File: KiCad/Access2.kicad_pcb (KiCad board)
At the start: 2 copper layers, 50 x 26.5 mm, 65 parts, among them J1 USB-C, J2 RFID, J3 INPUTS, J4 ExtTamper, J5 POWER, J6 DOOR, Q1 NX7002AK, SW1 Tamper, U1 ESP32-PICO-MINI-02, U2 FT231XQ, U3 G3VM-41GR8, U4 LMR16006+FB, U5 LMR16006+FB, U6 AA, U7 QR

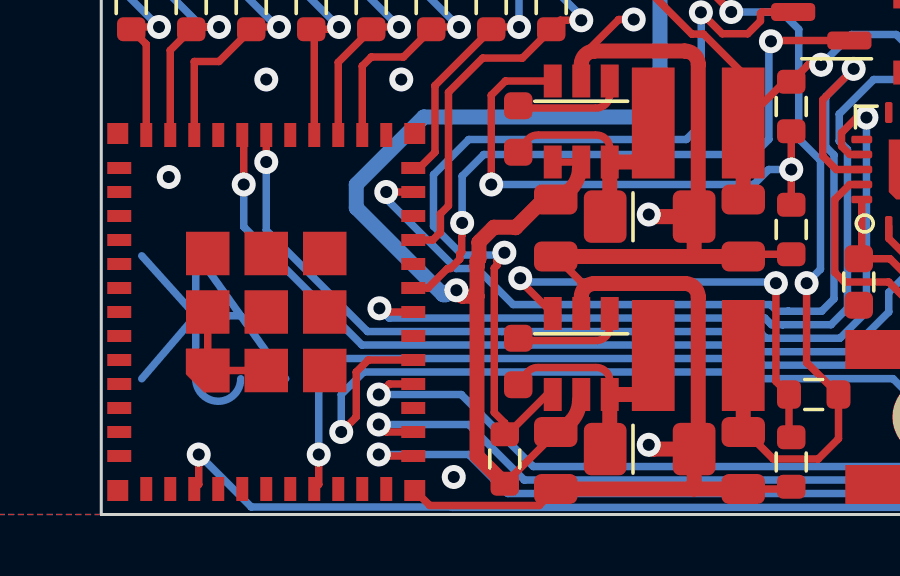
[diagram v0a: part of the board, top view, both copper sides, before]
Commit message: Tweak
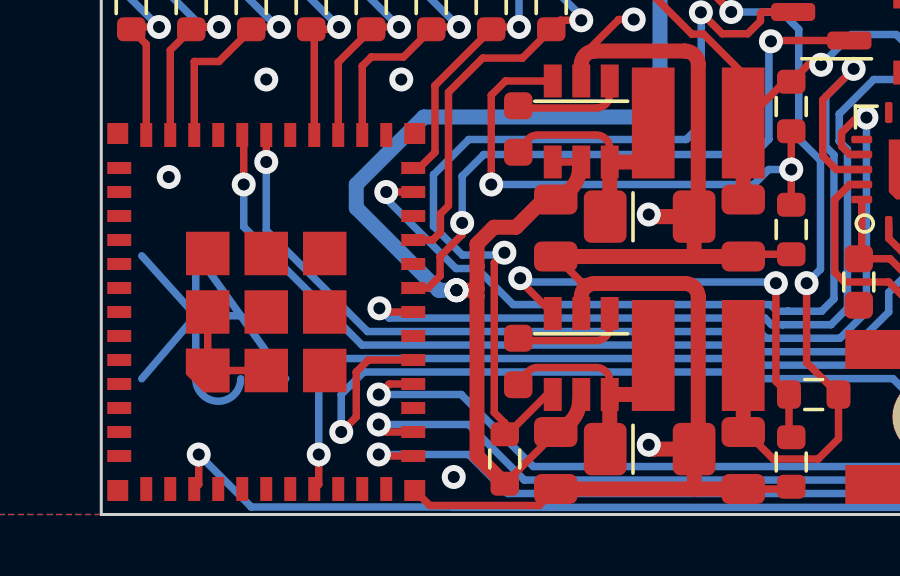
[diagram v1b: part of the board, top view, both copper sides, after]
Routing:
- net +12V: track 62.7 -> 62.5 mm, vias 1 -> 2
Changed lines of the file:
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@@
   (segment (start 128.620662 85.951956) (end 116.098352 85.951956) (width 0.25) (layer "B.Cu") (net 9))
   (segment (start 132.25 78) (end 131.098531 79.151469) (width 0.25) (layer "B.Cu") (net 9))
-  (segment (start 118.514852 83.746481) (end 118.514852 83.183896) (width 0.25) (layer "F.Cu") (net 10))
-  (segment (start 118.039296 84.300999) (end 118.136519 84.300999) (width 0.25) (layer "F.Cu") (net 10))
-  (segment (start 118.451458 83.809875) (end 118.514852 83.746481) (width 0.25) (layer "F.Cu") (net 10))
+  (segment (start 118.529927 82.779927) (end 118.529927 83.168821) (width 0.25) (layer "F.Cu") (net 10))
   (segment (start 131.4375 76.7) (end 128.849198 76.7) (width 0.25) (layer "F.Cu") (net 10))
-  (segment (start 118.451458 83.98606) (end 118.451458 83.809875) (width 0.25) (layer "F.Cu") (net 10))
-  (segment (start 116.9 84.95) (end 117.390295 84.95) (width 0.25) (layer "F.Cu") (net 10))
-  (segment (start 118.136519 84.300999) (end 118.451458 83.98606) (width 0.25) (layer "F.Cu") (net 10))
-  (segment (start 118.514852 83.183896) (end 118.529927 83.168821) (width 0.25) (layer "F.Cu") (net 10))
+  (segment (start 117.390295 84.95) (end 116.9 84.95) (width 0.25) (layer "F.Cu") (net 10))
   (segment (start 128.849198 76.7) (end 128.822959 76.726239) (width 0.25) (layer "F.Cu") (net 10))
-  (segment (start 118.529927 83.168821) (end 118.529927 82.779927) (width 0.25) (layer "F.Cu") (net 10))
-  (segment (start 117.390295 84.95) (end 118.039296 84.300999) (width 0.25) (layer "F.Cu") (net 10))
+  (segment (start 117.795148 84.545148) (end 117.390295 84.95) (width 0.25) (layer "F.Cu") (net 10))
+  (segment (start 117.795148 83.9036) (end 117.795148 84.545148) (width 0.25) (layer "F.Cu") (net 10))
+  (segment (start 118.529927 83.168821) (end 117.795148 83.9036) (width 0.25) (layer "F.Cu") (net 10))
   (via (at 128.822959 76.726239) (size 0.8) (drill 0.4) (layers "F.Cu" "B.Cu") (net 10))
   (via (at 118.529927 82.779927) (size 0.8) (drill 0.4) (layers "F.Cu" "B.Cu") (net 10))
@@
   (segment (start 131.727456 87.522544) (end 132.75 86.5) (width 0.25) (layer "B.Cu") (net 16))
   (segment (start 113.75 88) (end 114.44951 87.30049) (width 0.25) (layer "B.Cu") (net 16))
-  (segment (start 119.089363 83.984452) (end 119.025969 84.047846) (width 0.5) (layer "F.Cu") (net 17))
-  (segment (start 119.586988 82.924242) (end 119.089363 83.421867) (width 0.5) (layer "F.Cu") (net 17))
+  (segment (start 119.02548 84.97452) (end 119.02548 85.22452) (width 0.5) (layer "F.Cu") (net 17))
   (segment (start 142 76.75) (end 143.5125 76.75) (width 0.5) (layer "F.Cu") (net 17))
-  (segment (start 121.25 82) (end 120.308249 82.941751) (width 0.5) (layer "F.Cu") (net 17))
   (segment (start 143.5125 76.75) (end 144.7625 75.5) (width 0.5) (layer "F.Cu") (net 17))
-  (segment (start 119.02548 84.22452) (end 119.02548 85.22452) (width 0.5) (layer "F.Cu") (net 17))
-  (segment (start 118.538415 85.22452) (end 118.339395 85.0255) (width 0.5) (layer "F.Cu") (net 17))
+  (segment (start 119.025969 83.485261) (end 119.025969 84.224031) (width 0.5) (layer "F.Cu") (net 17))
+  (segment (start 118.339395 85.0255) (end 118.9745 85.0255) (width 0.5) (layer "F.Cu") (net 17))
+  (segment (start 120.325758 82.924242) (end 119.586988 82.924242) (width 0.5) (layer "F.Cu") (net 17))
+  (segment (start 119.586988 82.924242) (end 119.025969 83.485261) (width 0.5) (layer "F.Cu") (net 17))
+  (segment (start 118.9745 85.0255) (end 119.02548 84.97452) (width 0.5) (layer "F.Cu") (net 17))
+  (segment (start 119.025969 84.224031) (end 119.02548 84.22452) (width 0.5) (layer "F.Cu") (net 17))
   (segment (start 121.65 89.775) (end 119.95 91.475) (width 0.25) (layer "F.Cu") (net 17))
-  (segment (start 119.025969 84.224031) (end 119.02548 84.22452) (width 0.5) (layer "F.Cu") (net 17))
-  (segment (start 120.29074 82.924242) (end 119.586988 82.924242) (width 0.5) (layer "F.Cu") (net 17))
   (segment (start 121.65 82) (end 121.25 82) (width 0.5) (layer "F.Cu") (net 17))
   (segment (start 119.02548 90.55048) (end 119.95 91.475) (width 0.5) (layer "F.Cu") (net 17))
-  (segment (start 120.308249 82.941751) (end 120.29074 82.924242) (width 0.5) (layer "F.Cu") (net 17))
   (segment (start 121.55 80.75) (end 122.5 80.75) (width 0.25) (layer "F.Cu") (net 17))
   (segment (start 119.02548 85.22452) (end 119.02548 90.55048) (width 0.5) (layer "F.Cu") (net 17))
-  (segment (start 119.02548 85.22452) (end 118.538415 85.22452) (width 0.5) (layer "F.Cu") (net 17))
-  (segment (start 119.089363 83.421867) (end 119.089363 83.984452) (width 0.5) (layer "F.Cu") (net 17))
   (segment (start 121.65 89.75) (end 121.65 89.775) (width 0.25) (layer "F.Cu") (net 17))
-  (segment (start 119.025969 84.047846) (end 119.025969 84.224031) (width 0.5) (layer "F.Cu") (net 17))
+  (segment (start 119.02548 84.22452) (end 119.02548 84.97452) (width 0.5) (layer "F.Cu") (net 17))
+  (segment (start 121.25 82) (end 120.325758 82.924242) (width 0.5) (layer "F.Cu") (net 17))
   (via (at 118.339395 85.0255) (size 0.8) (drill 0.4) (layers "F.Cu" "B.Cu") (net 17))
+  (via (at 118.339395 85.0255) (size 0.8) (drill 0.4) (layers "F.Cu" "B.Cu") (net 17))
+  (segment (start 142 76.75) (end 138.562481 76.75) (width 0.5) (layer "B.Cu") (net 17))
+  (segment (start 124.5 79.25) (end 117.25 79.25) (width 0.5) (layer "B.Cu") (net 17))
+  (segment (start 125.5 74.75) (end 125.125 75.125) (width 0.5) (layer "B.Cu") (net 17))
+  (segment (start 144.5 75.08654) (end 142.83654 76.75) (width 0.5) (layer "B.Cu") (net 17))
+  (segment (start 115 81.5) (end 115 82.277518) (width 0.5) (layer "B.Cu") (net 17))
+  (segment (start 142.83654 76.75) (end 142 76.75) (width 0.5) (layer "B.Cu") (net 17))
+  (segment (start 117.747982 85.0255) (end 118.339395 85.0255) (width 0.5) (layer "B.Cu") (net 17))
+  (segment (start 136.562481 74.75) (end 125.5 74.75) (width 0.5) (layer "B.Cu") (net 17))
   (segment (start 138.562481 76.75) (end 136.562481 74.75) (width 0.5) (layer "B.Cu") (net 17))
-  (segment (start 124.5 79.25) (end 117.25 79.25) (width 0.5) (layer "B.Cu") (net 17))
-  (segment (start 117.897971 85.175489) (end 117.987971 85.175489) (width 0.5) (layer "B.Cu") (net 17))
-  (segment (start 117.987971 85.175489) (end 118.13796 85.0255) (width 0.5) (layer "B.Cu") (net 17))
+  (segment (start 115 82.277518) (end 117.747982 85.0255) (width 0.5) (layer "B.Cu") (net 17))
+  (segment (start 125.125 75.125) (end 125.125 78.625) (width 0.5) (layer "B.Cu") (net 17))
+  (segment (start 117.25 79.25) (end 115 81.5) (width 0.5) (layer "B.Cu") (net 17))
   (segment (start 125.125 78.625) (end 124.5 79.25) (width 0.5) (layer "B.Cu") (net 17))
-  (segment (start 144.5 75.08654) (end 142.83654 76.75) (width 0.5) (layer "B.Cu") (net 17))
-  (segment (start 118.13796 85.0255) (end 118.339395 85.0255) (width 0.5) (layer "B.Cu") (net 17))
-  (segment (start 142.83654 76.75) (end 142 76.75) (width 0.5) (layer "B.Cu") (net 17))
-  (segment (start 115 81.5) (end 115 82.277518) (width 0.5) (layer "B.Cu") (net 17))
-  (segment (start 125.5 74.75) (end 125.125 75.125) (width 0.5) (layer "B.Cu") (net 17))
-  (segment (start 115 82.277518) (end 117.897971 85.175489) (width 0.5) (layer "B.Cu") (net 17))
-  (segment (start 125.125 75.125) (end 125.125 78.625) (width 0.5) (layer "B.Cu") (net 17))
-  (segment (start 142 76.75) (end 138.562481 76.75) (width 0.5) (layer "B.Cu") (net 17))
-  (segment (start 117.25 79.25) (end 115 81.5) (width 0.5) (layer "B.Cu") (net 17))
-  (segment (start 136.562481 74.75) (end 125.5 74.75) (width 0.5) (layer "B.Cu") (net 17))
   (segment (start 144.5 72.65) (end 144.5 75.08654) (width 0.5) (layer "B.Cu") (net 17))
   (segment (start 139.80049 82.186194) (end 139.80049 80.97549) (width 0.25) (layer "F.Cu") (net 18))
@@
   (segment (start 128.050099 76.474501) (end 127.199901 76.474501) (width 0.25) (layer "F.Cu") (net 24))
   (segment (start 127.199901 76.474501) (end 126.487701 75.762299) (width 0.25) (layer "F.Cu") (net 24))
-  (segment (start 119.60048 89.10048) (end 119.60048 84.285816) (width 0.25) (layer "F.Cu") (net 24))
+  (segment (start 119.60048 89.10048) (end 119.95 89.45) (width 0.25) (layer "F.Cu") (net 24))
   (segment (start 121.55 88.5) (end 121.362507 88.5) (width 0.25) (layer "F.Cu") (net 24))
+  (segment (start 119.95 89.45) (end 119.95 89.825) (width 0.25) (layer "F.Cu") (net 24))
+  (segment (start 119.60048 84.112127) (end 119.60048 89.10048) (width 0.25) (layer "F.Cu") (net 24))
   (segment (start 120.037507 89.825) (end 119.95 89.825) (width 0.25) (layer "F.Cu") (net 24))
-  (segment (start 119.692713 84.019894) (end 119.938864 83.773743) (width 0.25) (layer "F.Cu") (net 24))
-  (segment (start 119.692713 84.193583) (end 119.692713 84.019894) (width 0.25) (layer "F.Cu") (net 24))
-  (segment (start 119.95 89.45) (end 119.60048 89.10048) (width 0.25) (layer "F.Cu") (net 24))
   (segment (start 128.474501 75.800099) (end 128.474501 76.050099) (width 0.25) (layer "F.Cu") (net 24))
   (segment (start 128.5246 75.75) (end 128.474501 75.800099) (width 0.25) (layer "F.Cu") (net 24))
   (segment (start 129.5625 75.75) (end 128.5246 75.75) (width 0.25) (layer "F.Cu") (net 24))
+  (segment (start 119.938864 83.773743) (end 119.60048 84.112127) (width 0.25) (layer "F.Cu") (net 24))
   (segment (start 121.362507 88.5) (end 120.037507 89.825) (width 0.25) (layer "F.Cu") (net 24))
   (segment (start 128.474501 76.050099) (end 128.050099 76.474501) (width 0.25) (layer "F.Cu") (net 24))
-  (segment (start 119.60048 84.285816) (end 119.692713 84.193583) (width 0.25) (layer "F.Cu") (net 24))
-  (segment (start 119.95 89.825) (end 119.95 89.45) (width 0.25) (layer "F.Cu") (net 24))
   (via (at 126.487701 75.762299) (size 0.8) (drill 0.4) (layers "F.Cu" "B.Cu") (net 24))
   (via (at 119.938864 83.773743) (size 0.8) (drill 0.4) (layers "F.Cu" "B.Cu") (net 24))

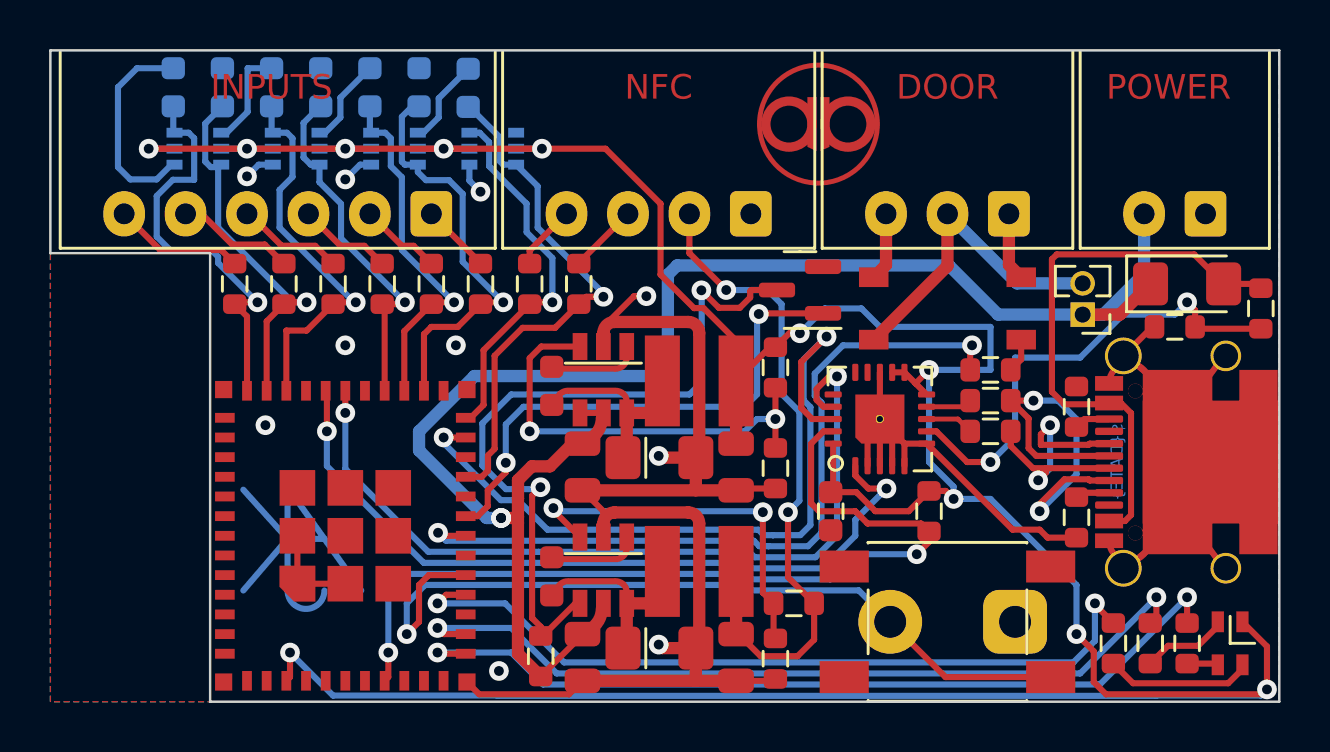
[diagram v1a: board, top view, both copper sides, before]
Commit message: Curvy tracks
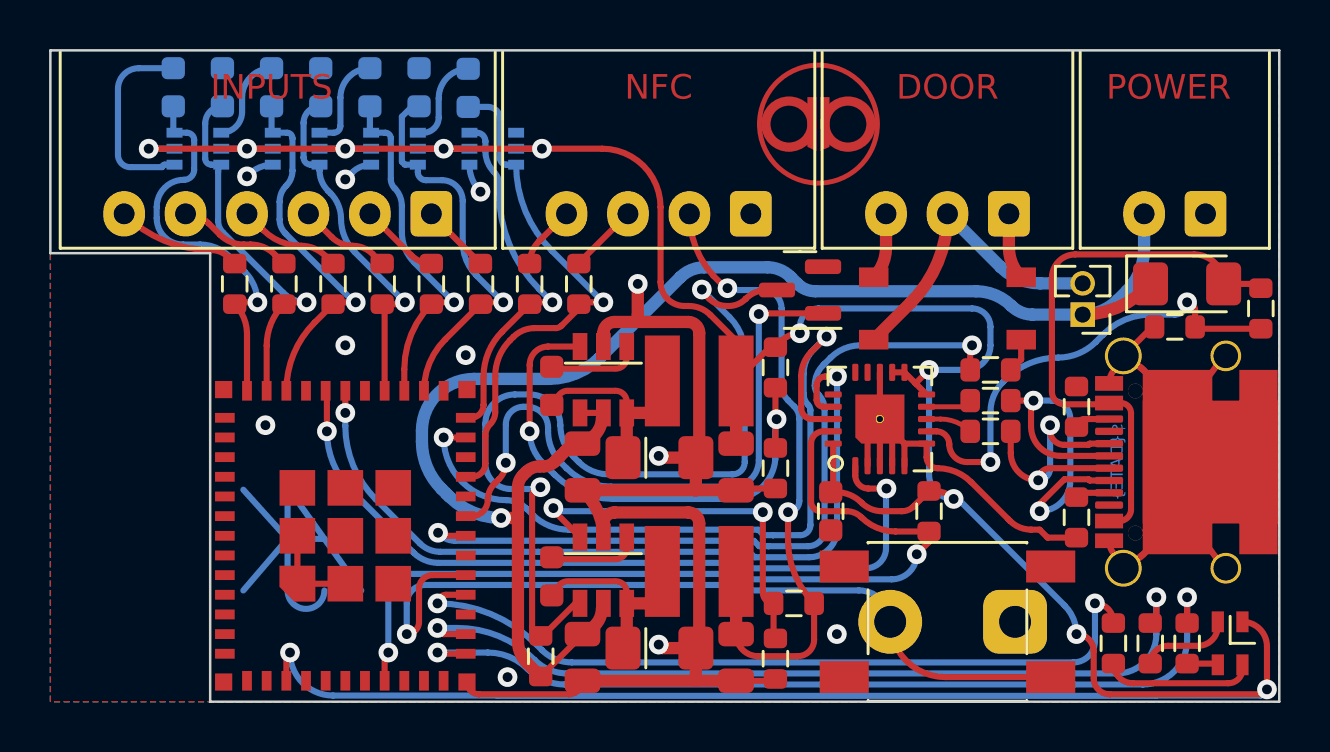
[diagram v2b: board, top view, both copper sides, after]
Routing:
- net Net-(Q1-Pad3): track 30.2 -> 37.3 mm
- net SHDN: track 21.3 -> 26.1 mm
- net Net-(R22-Pad2): track 17.9 -> 21.4 mm
- net +12V: track 62.5 -> 59.5 mm, vias 2 -> 1
- net GND: track 67.4 -> 65.3 mm, vias 10 -> 11
- net G: track 34.7 -> 35.8 mm
- net O: track 31.2 -> 32.1 mm
- net IN1: track 17.1 -> 16.2 mm
- net Net-(J1-PadA7): track 16.6 -> 15.7 mm
- net B: track 33.7 -> 34.5 mm
- net IN4: track 16.0 -> 15.2 mm
- net IN6: track 17.2 -> 16.6 mm
- net Net-(J1-PadA6): track 11.8 -> 11.2 mm
- net TAMPER: track 33.6 -> 34.1 mm
- net Net-(R2-Pad2): track 19.6 -> 19.0 mm
